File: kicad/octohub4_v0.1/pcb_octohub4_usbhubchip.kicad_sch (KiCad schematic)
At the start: 43 parts, among them J301 USB_C_Receptacle_USB2.0, U301 AMS1117-3.3, U302 USB2514B_Bi, Y301 24MHz

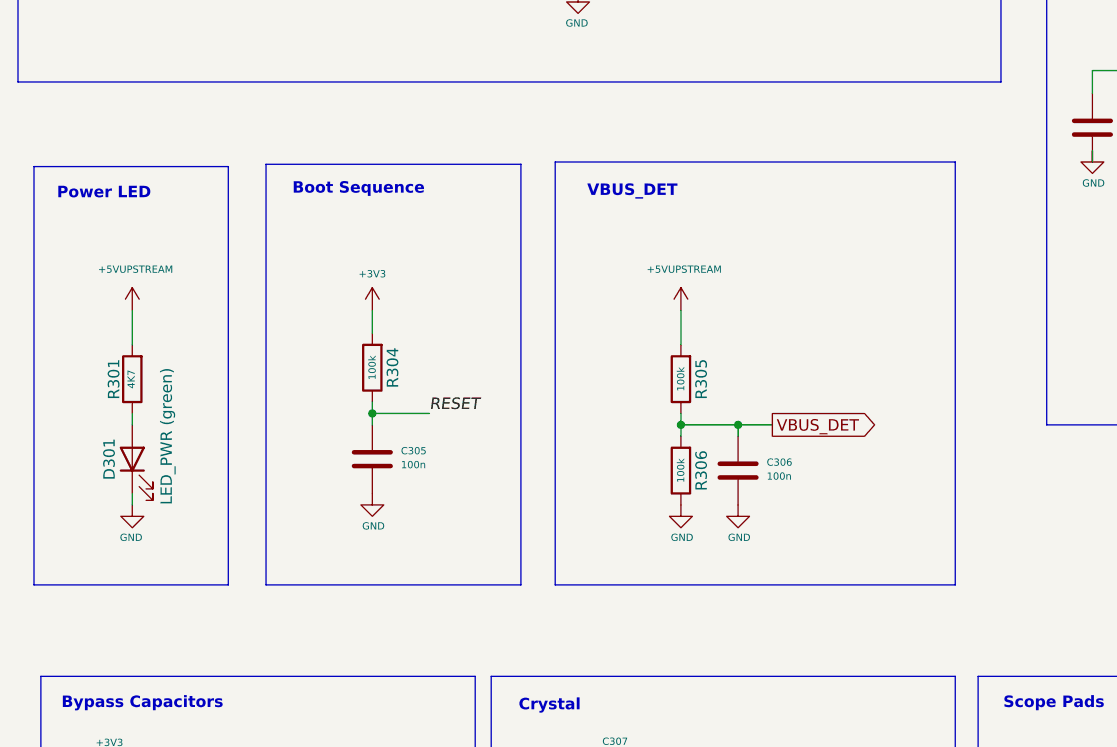
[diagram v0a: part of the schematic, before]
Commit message: Add run_kicad_purge 3
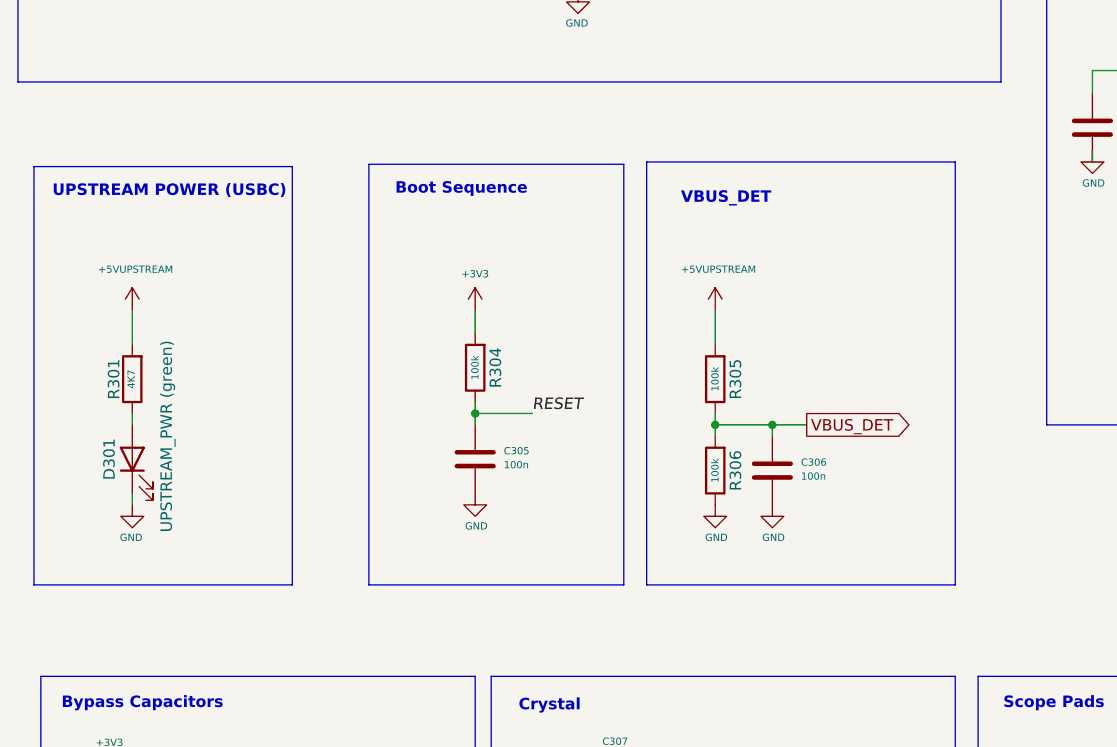
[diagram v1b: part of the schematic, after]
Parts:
- D301: Label LED_PWR (green) -> UPSTREAM_PWR (green)
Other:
- note added: "UPSTREAM POWER (USBC)"
- note removed: "Power LED"
- moved on the sheet: C305, C306, R304, R305, R306

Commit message: New via constraints: Copy usb hub footprint from tentacle v0.7
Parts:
- U302: footprint Package_DFN_QFN:Texas_RHH0036C_VQFN-36-1EP_6x6mm_P0.5mm_EP4.4x4.4mm_ThermalVias -> 00_project_library:Texas_RHH0036C_VQFN-36-1EP_6x6mm_P0.5mm_EP4.4x4.4mm_ThermalVias
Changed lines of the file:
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@@
 			)
 		)
-		(property "Footprint" "Package_DFN_QFN:Texas_RHH0036C_VQFN-36-1EP_6x6mm_P0.5mm_EP4.4x4.4mm_ThermalVias"
+		(property "Footprint" "00_project_library:Texas_RHH0036C_VQFN-36-1EP_6x6mm_P0.5mm_EP4.4x4.4mm_ThermalVias"
 			(at 245.11 114.3 0)
 			(effects
